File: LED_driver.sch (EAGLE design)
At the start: 17 parts

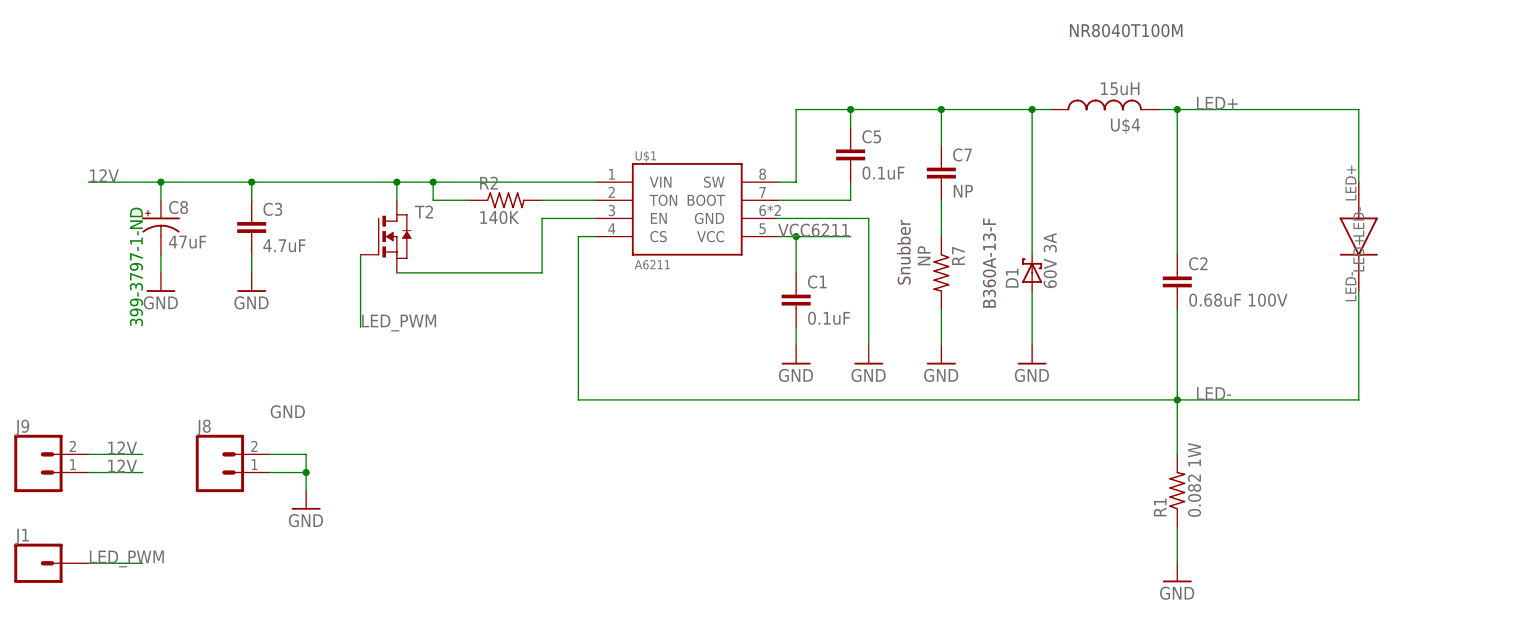
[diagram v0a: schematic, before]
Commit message: continued revisions
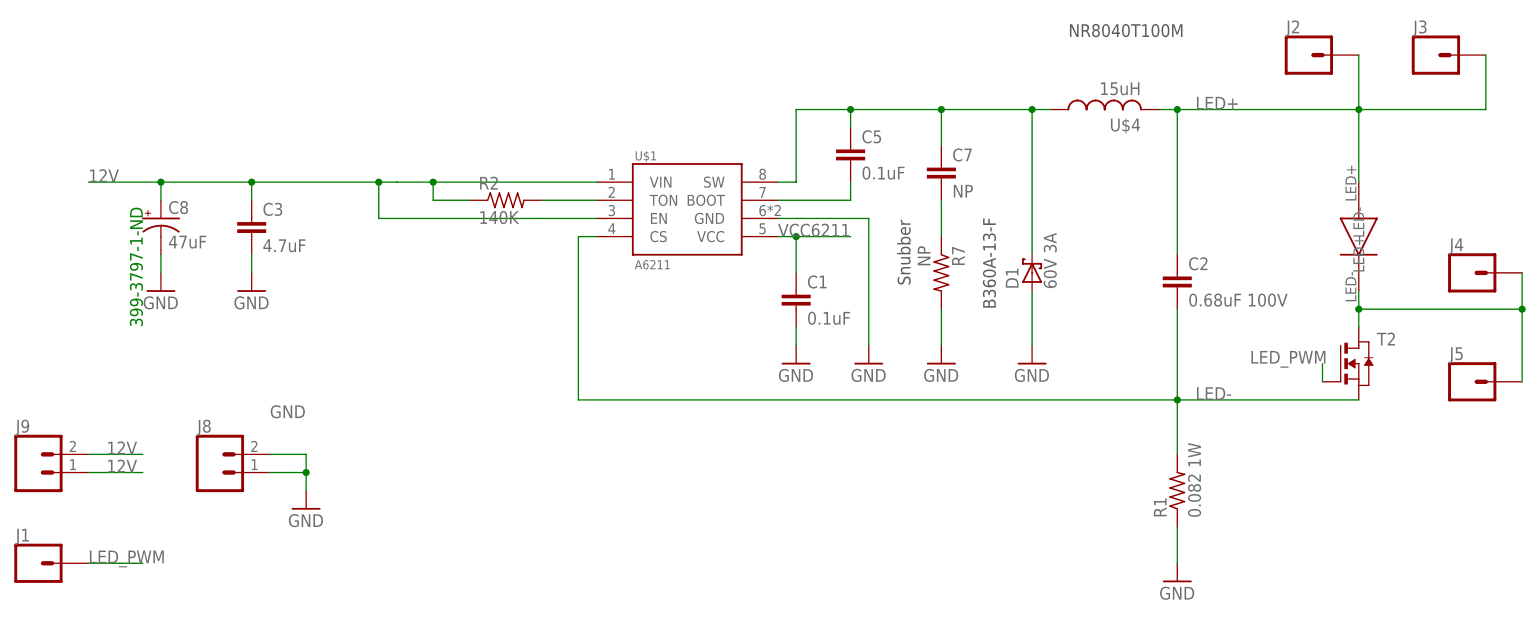
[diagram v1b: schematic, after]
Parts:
- added J2, J3, J4, J5: (no value), SparkFun-Connectors:CONN_01
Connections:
- removed net N$7: T2.S, U$1.EN
- new net N$3: J4.1, J5.1, T2.D, U$3.LED-
- net 12V: now also U$1.EN; no longer T2.D
- net LED+: now also J2.1, J3.1
- net LED-: now also T2.S; no longer U$3.LED-
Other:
- moved on the sheet: T2
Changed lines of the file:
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@@
 <layer number="2" name="Route2" color="1" fill="3" visible="no" active="no"/>
 <layer number="3" name="Route3" color="4" fill="3" visible="no" active="no"/>
+<layer number="4" name="Route4" color="1" fill="4" visible="no" active="no"/>
+<layer number="5" name="Route5" color="4" fill="4" visible="no" active="no"/>
+<layer number="6" name="Route6" color="1" fill="8" visible="no" active="no"/>
+<layer number="7" name="Route7" color="4" fill="8" visible="no" active="no"/>
+<layer number="8" name="Route8" color="1" fill="2" visible="no" active="no"/>
+<layer number="9" name="Route9" color="4" fill="2" visible="no" active="no"/>
+<layer number="10" name="Route10" color="1" fill="7" visible="no" active="no"/>
+<layer number="11" name="Route11" color="4" fill="7" visible="no" active="no"/>
+<layer number="12" name="Route12" color="1" fill="5" visible="no" active="no"/>
+<layer number="13" name="Route13" color="4" fill="5" visible="no" active="no"/>
 <layer number="14" name="Route14" color="1" fill="6" visible="no" active="no"/>
 <layer number="15" name="Route15" color="4" fill="6" visible="no" active="no"/>
@@
 <part name="U$3" library="LED_00H53" deviceset="LED_00H53" device=""/>
 <part name="T2" library="zetex" deviceset="NMOSSOT23" device=""/>
+<part name="J2" library="SparkFun-Connectors" library_urn="urn:adsk.eagle:library:513" deviceset="CONN_01" device="" package3d_urn="urn:adsk.eagle:package:38028/1"/>
+<part name="J3" library="SparkFun-Connectors" library_urn="urn:adsk.eagle:library:513" deviceset="CONN_01" device="" package3d_urn="urn:adsk.eagle:package:38028/1"/>
+<part name="J4" library="SparkFun-Connectors" library_urn="urn:adsk.eagle:library:513" deviceset="CONN_01" device="" package3d_urn="urn:adsk.eagle:package:38028/1"/>
+<part name="J5" library="SparkFun-Connectors" library_urn="urn:adsk.eagle:library:513" deviceset="CONN_01" device="" package3d_urn="urn:adsk.eagle:package:38028/1"/>
 </parts>
 <sheets>
@@
 <instance part="J9" gate="G$1" x="45.72" y="81.28"/>
 <instance part="U$3" gate="G$1" x="231.14" y="114.3" rot="R270"/>
-<instance part="T2" gate="A" x="96.52" y="114.3"/>
+<instance part="T2" gate="A" x="231.14" y="96.52"/>
+<instance part="J2" gate="G$1" x="223.52" y="139.7"/>
+<instance part="J3" gate="G$1" x="241.3" y="139.7"/>
+<instance part="J4" gate="G$1" x="246.38" y="109.22"/>
+<instance part="J5" gate="G$1" x="246.38" y="93.98"/>
 </instances>
 <busses>
@@
 <wire x1="124.46" y1="121.92" x2="101.6" y2="121.92" width="0.1524" layer="91"/>
 <wire x1="101.6" y1="121.92" x2="96.52" y2="121.92" width="0.1524" layer="91"/>
-<wire x1="96.52" y1="121.92" x2="76.2" y2="121.92" width="0.1524" layer="91"/>
+<wire x1="96.52" y1="121.92" x2="93.98" y2="121.92" width="0.1524" layer="91"/>
+<wire x1="93.98" y1="121.92" x2="76.2" y2="121.92" width="0.1524" layer="91"/>
 <wire x1="76.2" y1="121.92" x2="63.5" y2="121.92" width="0.1524" layer="91"/>
 <wire x1="63.5" y1="121.92" x2="53.34" y2="121.92" width="0.1524" layer="91"/>
@@
 <junction x="63.5" y="121.92"/>
 <pinref part="C3" gate="G$1" pin="1"/>
-<pinref part="T2" gate="A" pin="D"/>
-<wire x1="96.52" y1="119.38" x2="96.52" y2="121.92" width="0.1524" layer="91"/>
-<junction x="96.52" y="121.92"/>
+<pinref part="U$1" gate="G$1" pin="EN"/>
+<wire x1="116.84" y1="116.84" x2="124.46" y2="116.84" width="0.1524" layer="91"/>
+<wire x1="116.84" y1="116.84" x2="93.98" y2="116.84" width="0.1524" layer="91"/>
+<wire x1="93.98" y1="116.84" x2="93.98" y2="121.92" width="0.1524" layer="91"/>
+<junction x="93.98" y="121.92"/>
 </segment>
 <segment>
@@
 <wire x1="205.74" y1="132.08" x2="231.14" y2="132.08" width="0.1524" layer="91"/>
 <wire x1="231.14" y1="132.08" x2="231.14" y2="121.92" width="0.1524" layer="91"/>
+<pinref part="J2" gate="G$1" pin="1"/>
+<wire x1="231.14" y1="132.08" x2="231.14" y2="139.7" width="0.1524" layer="91"/>
+<junction x="231.14" y="132.08"/>
+<pinref part="J3" gate="G$1" pin="1"/>
+<wire x1="231.14" y1="132.08" x2="248.92" y2="132.08" width="0.1524" layer="91"/>
+<wire x1="248.92" y1="132.08" x2="248.92" y2="139.7" width="0.1524" layer="91"/>
 </segment>
 </net>
@@
 <wire x1="121.92" y1="114.3" x2="124.46" y2="114.3" width="0.1524" layer="91"/>
 <label x="208.28" y="91.44" size="1.778" layer="95"/>
-<wire x1="231.14" y1="91.44" x2="205.74" y2="91.44" width="0.1524" layer="91"/>
-<pinref part="U$3" gate="G$1" pin="LED-"/>
-<wire x1="231.14" y1="91.44" x2="231.14" y2="106.68" width="0.1524" layer="91"/>
+<pinref part="T2" gate="A" pin="S"/>
+<wire x1="205.74" y1="91.44" x2="231.14" y2="91.44" width="0.1524" layer="91"/>
 </segment>
 </net>
@@
 <segment>
 <pinref part="T2" gate="A" pin="G"/>
-<wire x1="91.44" y1="111.76" x2="91.44" y2="101.6" width="0.1524" layer="91"/>
-<label x="91.44" y="101.6" size="1.778" layer="95"/>
-</segment>
-</net>
-<net name="N$7" class="0">
-<segment>
-<pinref part="T2" gate="A" pin="S"/>
-<wire x1="96.52" y1="109.22" x2="116.84" y2="109.22" width="0.1524" layer="91"/>
-<pinref part="U$1" gate="G$1" pin="EN"/>
-<wire x1="116.84" y1="109.22" x2="116.84" y2="116.84" width="0.1524" layer="91"/>
-<wire x1="116.84" y1="116.84" x2="124.46" y2="116.84" width="0.1524" layer="91"/>
-</segment>
-</net>
+<wire x1="226.06" y1="93.98" x2="226.06" y2="96.52" width="0.1524" layer="91"/>
+<label x="215.9" y="96.52" size="1.778" layer="95"/>
+</segment>
+</net>
+<net name="N$3" class="0">
+<segment>
+<pinref part="T2" gate="A" pin="D"/>
+<pinref part="U$3" gate="G$1" pin="LED-"/>
+<wire x1="231.14" y1="101.6" x2="231.14" y2="104.14" width="0.1524" layer="91"/>
+<pinref part="J4" gate="G$1" pin="1"/>
+<wire x1="231.14" y1="104.14" x2="231.14" y2="106.68" width="0.1524" layer="91"/>
+<wire x1="231.14" y1="104.14" x2="254" y2="104.14" width="0.1524" layer="91"/>
+<wire x1="254" y1="104.14" x2="254" y2="109.22" width="0.1524" layer="91"/>
+<junction x="231.14" y="104.14"/>
+<pinref part="J5" gate="G$1" pin="1"/>
+<wire x1="254" y1="93.98" x2="254" y2="104.14" width="0.1524" layer="91"/>
+<junction x="254" y="104.14"/>
+</segment>
+</net>
